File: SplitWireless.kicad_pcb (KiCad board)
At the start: 2 copper layers, 190.9 x 138.6 mm, 57 parts, among them J1 OLED_128x32, SW1 Switch, SW2 Push_Button, U2 Nice_Nano_V2

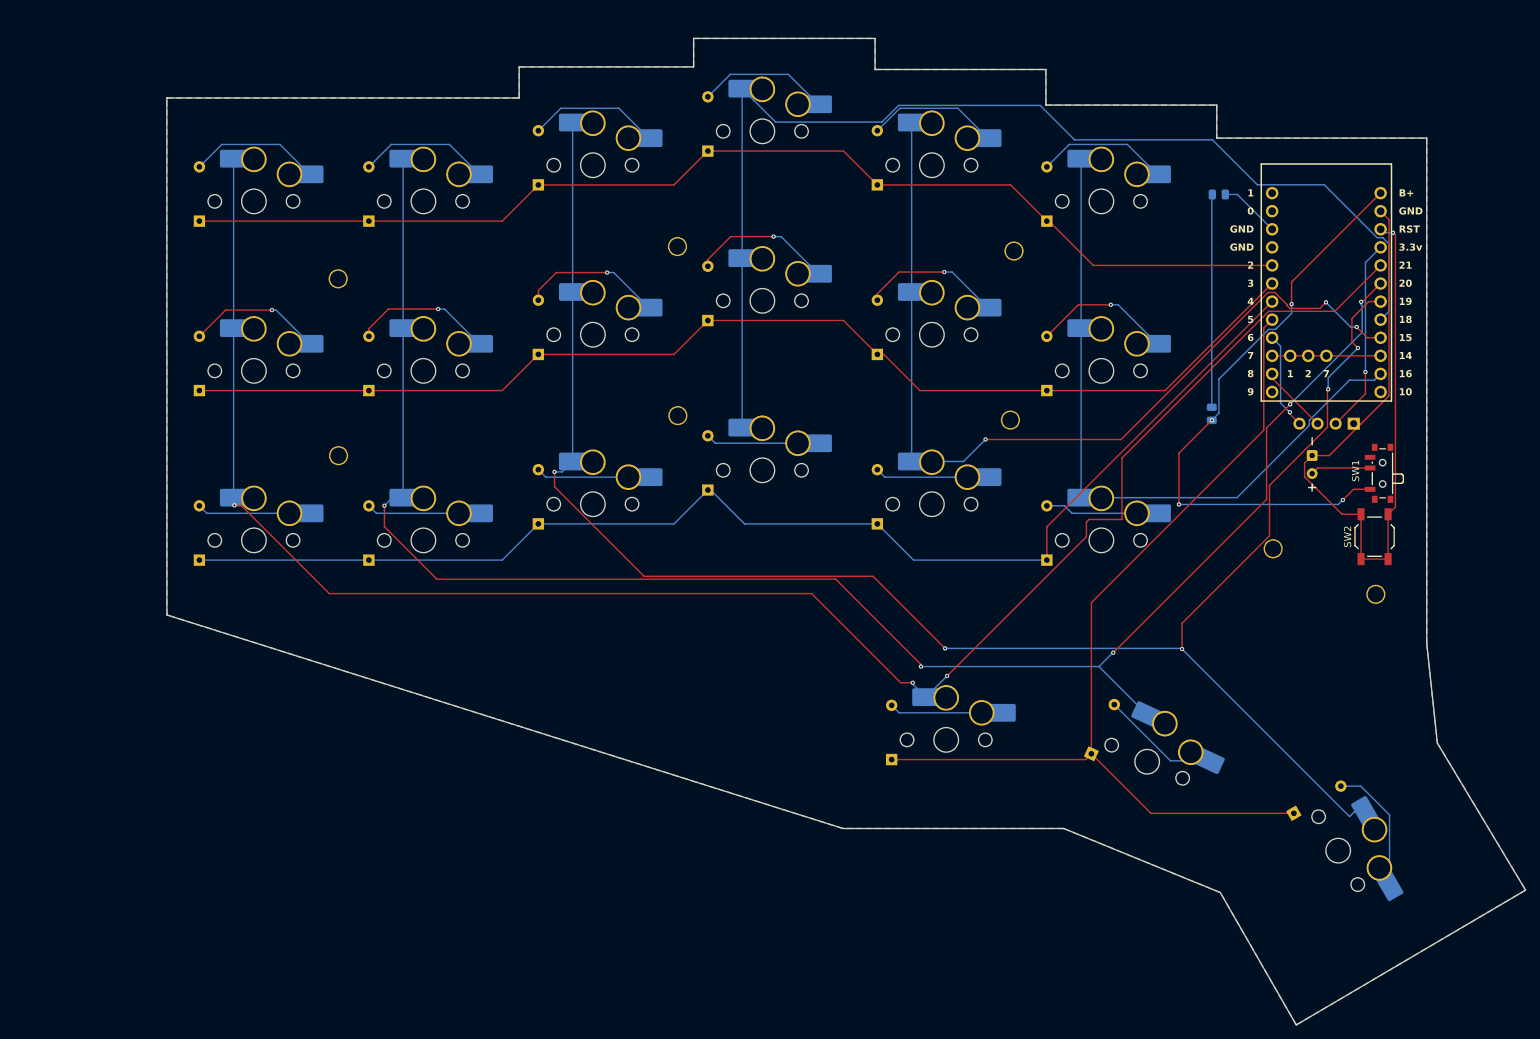
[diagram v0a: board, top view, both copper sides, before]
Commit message: added some stuff
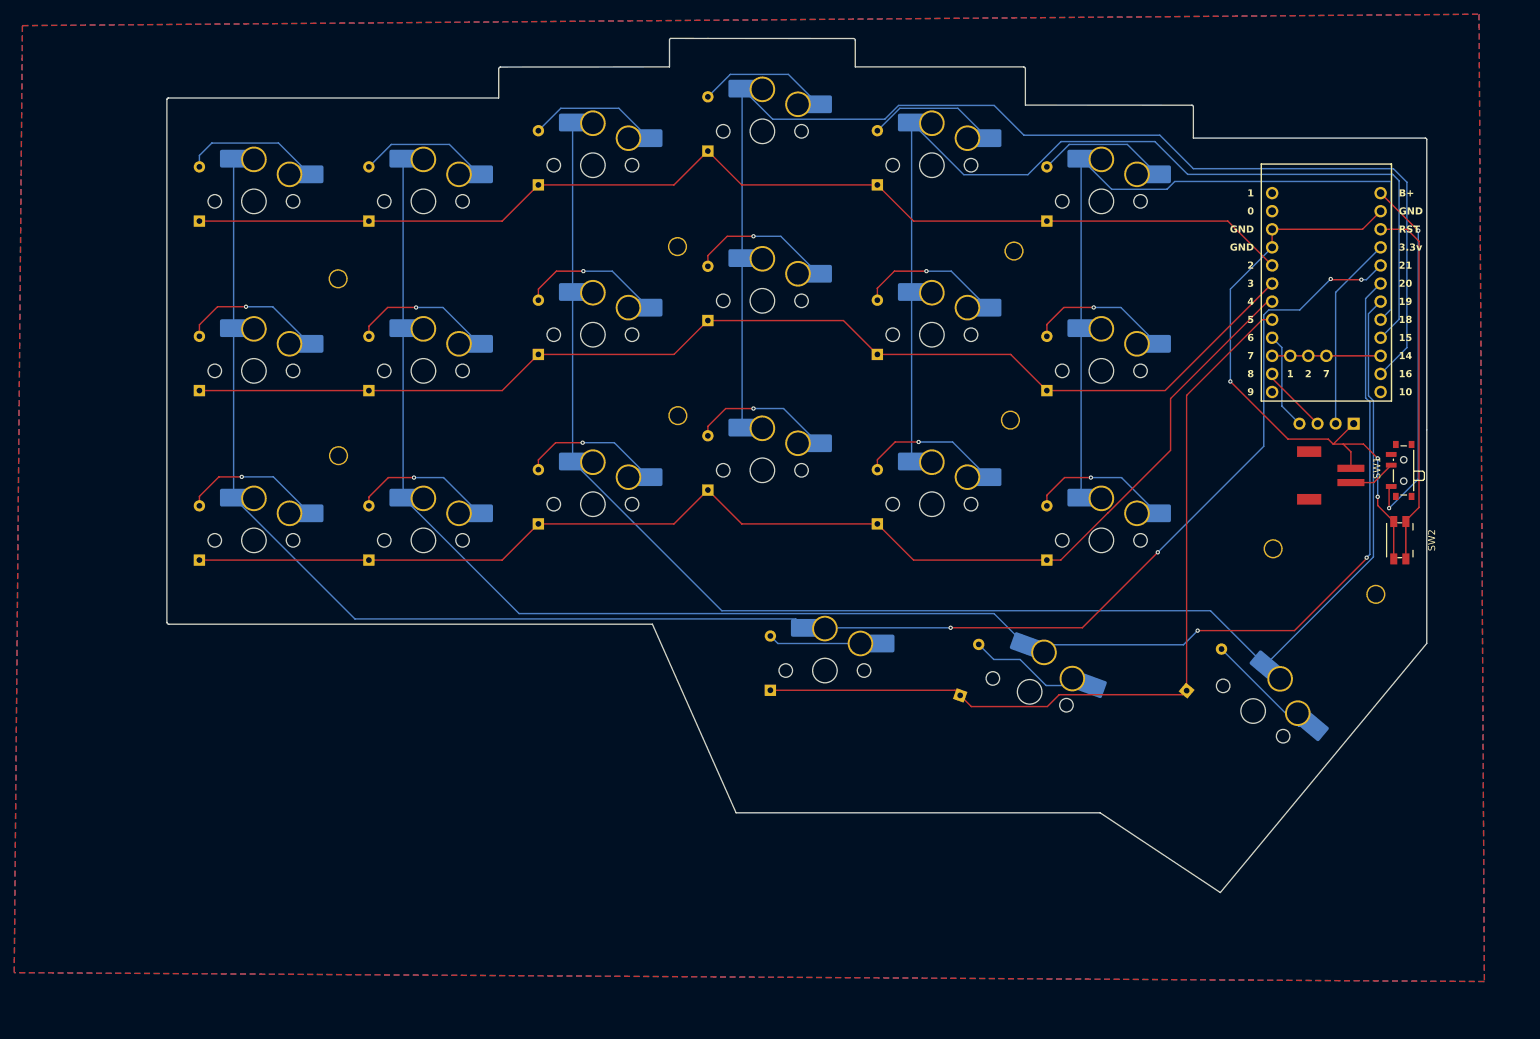
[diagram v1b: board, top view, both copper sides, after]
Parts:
- removed BT1: Battery, ScottoKeebs_Scotto:Battery
- removed R1: 1M, ScottoKeebs_Components:Resistor_0805
- removed R2: 470K, ScottoKeebs_Components:Resistor_0805
- added J3: Conn_01x02, ScottoKeebs_Components:Connector_1x02_JST-PH, F.Cu at (227.7, 77.8)
- SW2: footprint Button_Switch_SMD:SW_SPST_TL3342 -> Button_Switch_SMD:Panasonic_EVQPUJ_EVQPUA
- moved S19 24.8 mm to (221.9, 108.8), turned to -40 degrees
- moved D19 22.9 mm to (207.5, 108.0), turned to 50 degrees
- moved D20 20.2 mm to (175.7, 108.7), turned to 70 degrees
- moved S20 19.7 mm to (189.5, 104.5), turned to -20 degrees
- moved D21 19.6 mm to (149.1, 108.0)
- moved S21 19.6 mm to (159.2, 100.3)
- moved SW2 3.58 mm to (237.5, 86.9), turned to -90 degrees
- moved SW1 2.99 mm to (237.7, 77.1)
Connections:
- SW2 pad 1: gnd -> RST
- U2 pad 14: Col5 -> Col3
- U2 pad 17: Col3 -> Col5
- U2 pad 22: gnd -> RST
- U2 pad 3: Net-(R2-Pad2) -> gnd
- U2 pad 4: unconnected-(U2-GND-Pad4) -> gnd
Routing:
- net RST: track 0.00 -> 51.5 mm
- net Col2: track 248.2 -> 215.2 mm, vias 5 -> 0
- net Net-(U2-B+): track 83.8 -> 51.3 mm, vias 4 -> 2
- net Net-(R1-Pad2): track 29.9 -> 0.00 mm
- net gnd: track 113.7 -> 88.3 mm, vias 1 -> 3
- net Col4: track 126.8 -> 146.5 mm, vias 3 -> 0
- net Col5: track 97.3 -> 113.5 mm
- net Col3: track 160.6 -> 176.5 mm
- net Row3: track 131.8 -> 118.3 mm
- net Net-(R2-Pad2): track 8.61 -> 0.00 mm
- net Col1: track 242.4 -> 236.5 mm, vias 5 -> 2
- net Net-(D13-A): track 15.9 -> 20.1 mm, vias 0 -> 1
- net Net-(D18-A): track 15.9 -> 20.1 mm, vias 0 -> 1
- net Col0: track 252.4 -> 248.3 mm, vias 3 -> 4
- net Net-(D14-A): track 15.9 -> 20.0 mm, vias 0 -> 1
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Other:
- board size 190.9 x 138.6 mm -> 177 x 120 mm
